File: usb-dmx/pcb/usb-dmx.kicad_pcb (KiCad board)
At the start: 2 copper layers, 25 x 35 mm, 22 parts, among them J1 USB_C_Receptacle_USB2.0_16P, J2 USB_A, SW1 PTS526_SM15_SMTR2_LFS, U1 IP4234CZ6, U2 ADP2108AUJ-3.3, U3 ESP32-S3-MINI-1U, U4 ST485E

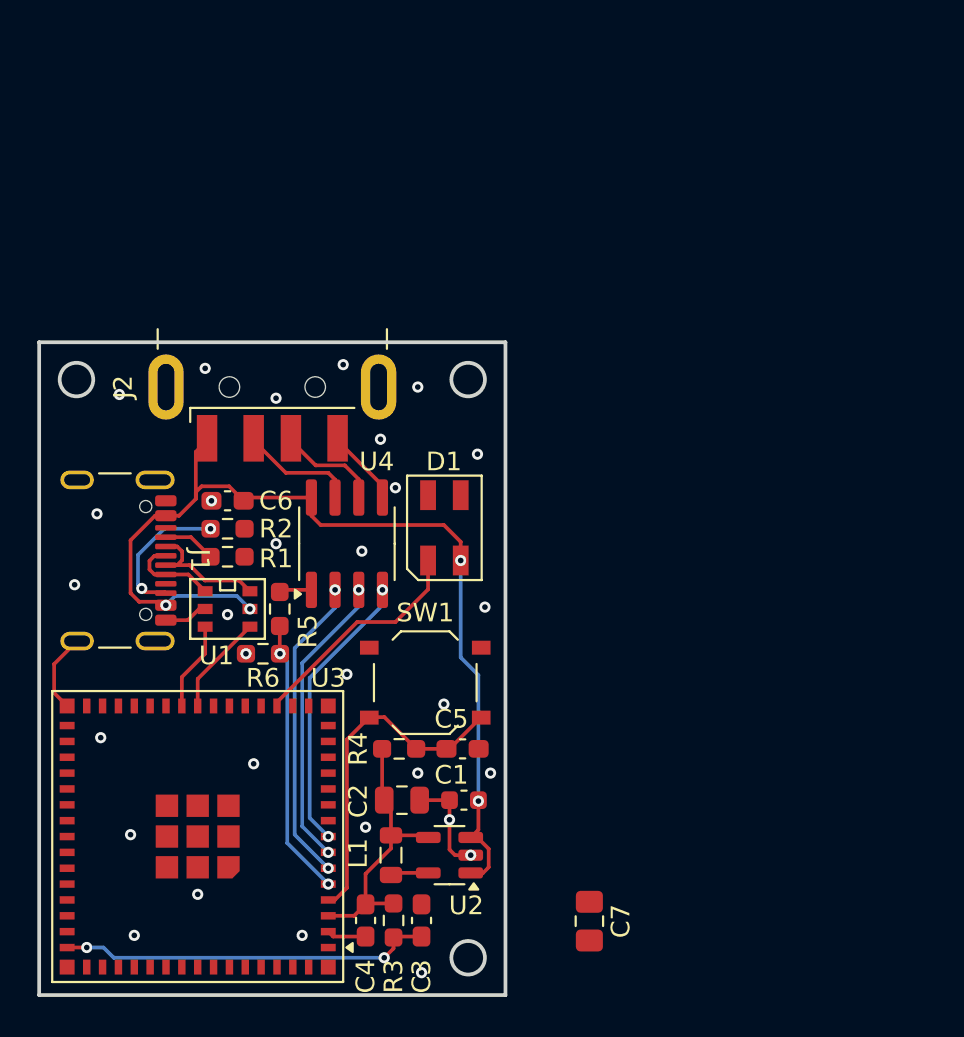
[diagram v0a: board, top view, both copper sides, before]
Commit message: creating pcb layout
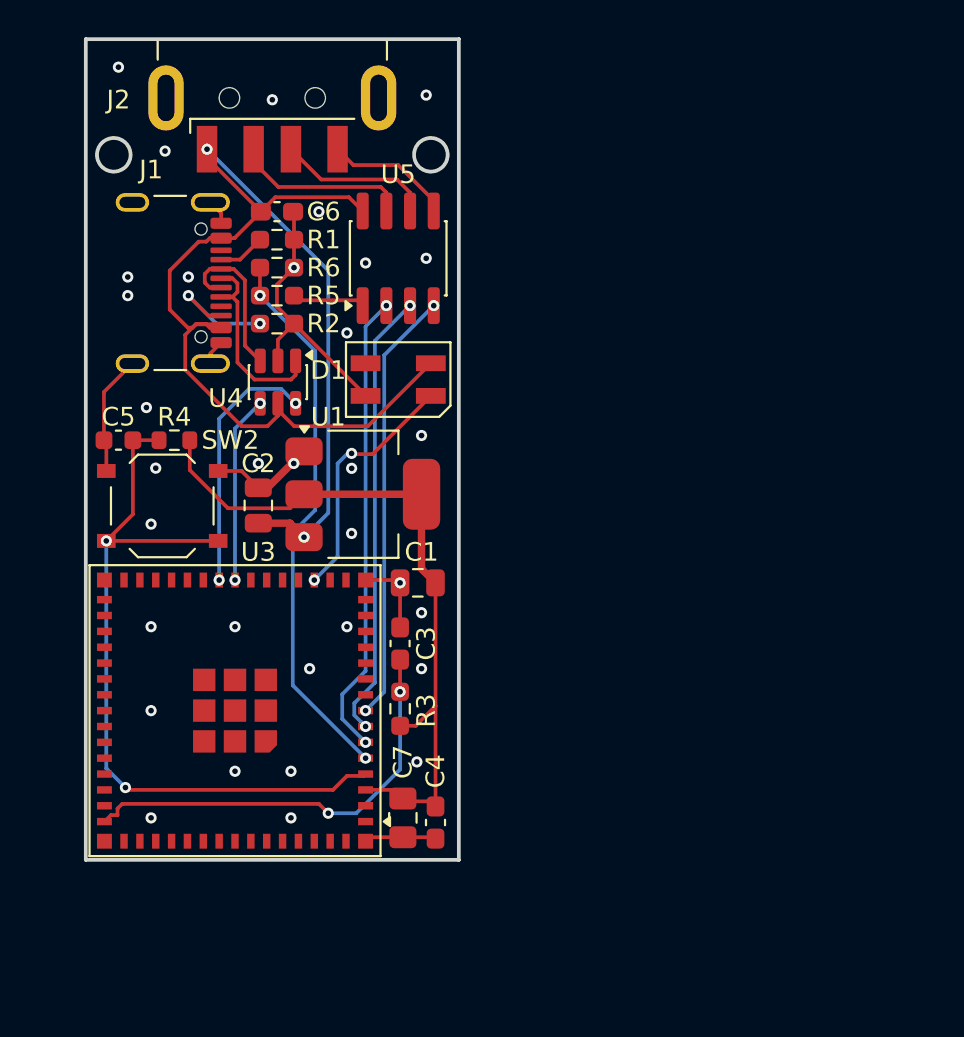
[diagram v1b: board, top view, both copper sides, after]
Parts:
- removed L1: 1uH, Inductor_SMD:L_0805_2012Metric
- removed SW1: PTS526_SM15_SMTR2_LFS, Button_Switch_SMD:SW_Push_1P1T_XKB_TS-1187A
- removed U2: ADP2108AUJ-3.3, Package_TO_SOT_SMD:TSOT-23-5
- added SW2: SW_Push, Button_Switch_SMD:SW_Push_1P1T_XKB_TS-1187A, F.Cu at (94.1, 68.8)
- added U5: MAX485E, Package_SO:SOP-8_3.76x4.96mm_P1.27mm, F.Cu at (106.8, 55.5)
- C1: value 4.7uF -> 22uF; footprint Capacitor_SMD:C_0603_1608Metric -> Capacitor_SMD:C_0805_2012Metric
- C2: value 10uF -> 22uF
- C5: footprint Capacitor_SMD:C_0603_1608Metric_Pad1.08x0.95mm_HandSolder -> Capacitor_SMD:C_0603_1608Metric
- R4: footprint Resistor_SMD:R_0603_1608Metric_Pad0.98x0.95mm_HandSolder -> Resistor_SMD:R_0603_1608Metric
- U1: value IP4234CZ6 -> AMS1117-3.3; footprint footprints:IP4234CZ6_SOT-457-6 -> Package_TO_SOT_SMD:SOT-223-3_TabPin2
- U4: value ST485E -> USBLC6-2SC6; footprint Package_SO:SOIC-8_3.9x4.9mm_P1.27mm -> Package_TO_SOT_SMD:SOT-23-6
- moved C5 24.8 mm to (91.8, 65.2), turned to 180 degrees
- moved R6 20.7 mm to (100.2, 56.0), turned to 0 degrees
- moved R4 20.5 mm to (94.8, 65.2), turned to 180 degrees
- moved C2 17.6 mm to (99.2, 68.8), turned to 90 degrees
- moved R1 17.2 mm to (100.2, 54.5)
- moved R5 16.8 mm to (100.2, 57.5), turned to 0 degrees
- moved C6 15.7 mm to (100.2, 53.0), turned to 0 degrees
- moved J2 15.5 mm to (100.0, 40.0)
- moved J1 15.2 mm to (93.6, 56.8)
- moved C3 14.9 mm to (106.8, 76.2)
- moved C1 11.9 mm to (107.8, 72.9)
- moved C7 11.4 mm to (107.0, 85.5)
- moved R3 11.4 mm to (106.8, 79.7), turned to 90 degrees
- moved R2 11.3 mm to (100.2, 59.0)
- moved U1 9.51 mm to (104.8, 68.2)
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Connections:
- C1 pad 1: VCC_5V -> VCC_3.3V
- C2 pad 1: VCC_3.3V -> VCC_5V
- R5 pad 2: Net-(U4-RO) -> Net-(U5-RO)
- U1 pad 1: Net-(J1-D+-PadA6) -> GND
- U1 pad 2: GND -> VCC_3.3V
- U1 pad 3: D+ -> VCC_5V
- U4 pad 1: Net-(U4-RO) -> Net-(J1-D+-PadA6)
- U4 pad 2: 2 -> GND
- U4 pad 3: 3 -> Net-(J1-D--PadA7)
- U4 pad 4: 4 -> D-
- U4 pad 5: GND -> VCC_5V
- U4 pad 6: DMX+ -> D+
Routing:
- net GND: track 18.3 -> 45.0 mm, vias 30 -> 33
- net VCC_3.3V: track 14.9 -> 38.7 mm
- net 0: track 18.3 -> 40.3 mm, vias 0 -> 2
- net VCC_5V: track 54.2 -> 70.6 mm, vias 4 -> 2
- net 1: track 14.9 -> 29.6 mm
- net D+: track 4.77 -> 13.7 mm, vias 0 -> 2
- net 2: track 16.6 -> 24.9 mm
- net 3: track 15.9 -> 24.0 mm
- net 4: track 15.3 -> 23.2 mm
- net Net-(J1-D+-PadA6): track 4.92 -> 10.4 mm
- net D-: track 5.41 -> 10.0 mm, vias 0 -> 2
- net Net-(U5-RO): track 0.00 -> 3.80 mm
- net Net-(U3-EN): track 20.0 -> 23.5 mm
- net DMX-: track 6.19 -> 9.48 mm
- net DMX+: track 5.47 -> 8.34 mm
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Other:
- board size 25 x 35 mm -> 20 x 44 mm
- board text added: "${REFERENCE}"
- board text added: "TRANCE USB-DMX Rev: 1.2"
- board text removed: "TRANCE USB-DMX Rev: 1.1"

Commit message: updating documentation
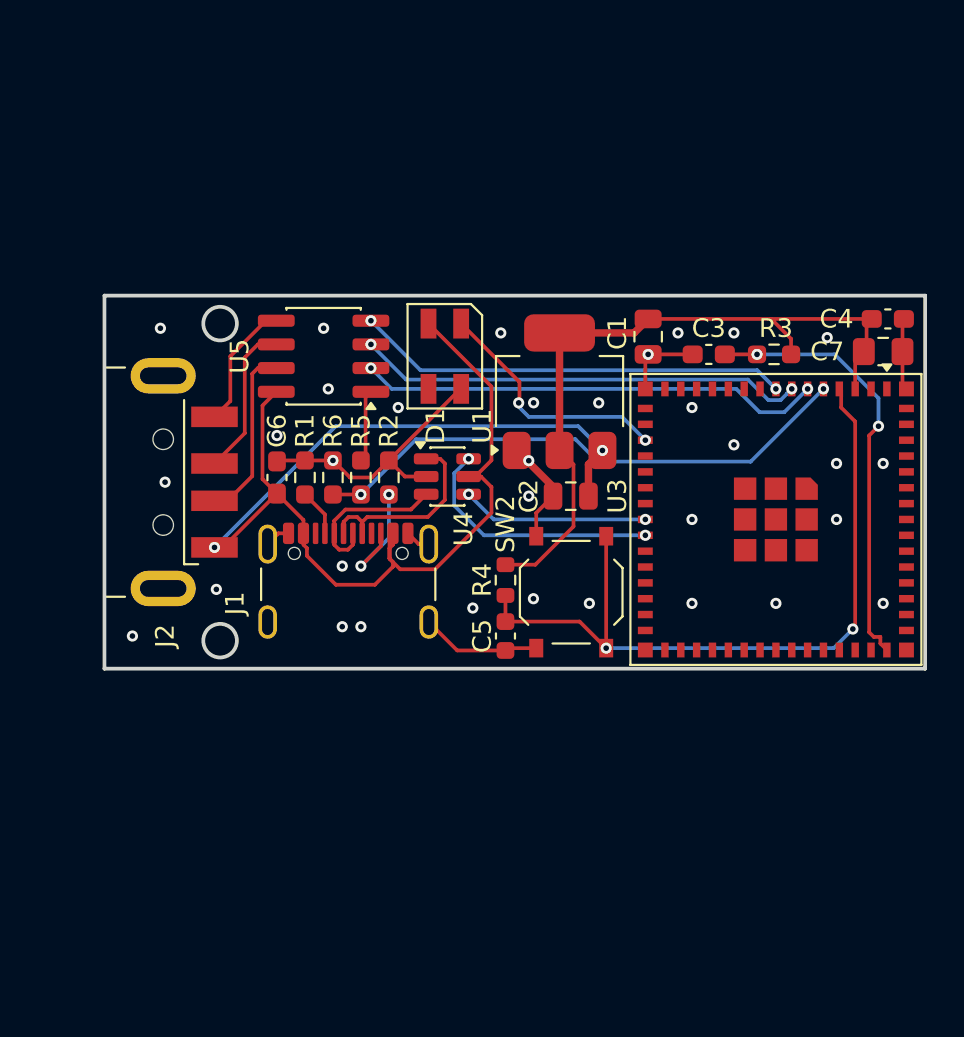
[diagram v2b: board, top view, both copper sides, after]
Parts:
- moved C4 36.3 mm to (133.0, 58.8), turned to 0 degrees
- moved C7 35.9 mm to (132.8, 60.5), turned to 0 degrees
- moved U3 30.8 mm to (127.0, 69.5), turned to -90 degrees
- moved J2 30.3 mm to (87.2, 67.5), turned to 180 degrees
- moved R3 27.6 mm to (126.9, 60.6), turned to 180 degrees
- moved C5 23.3 mm to (112.5, 75.8), turned to -90 degrees
- moved C3 22.7 mm to (123.4, 60.6), turned to 180 degrees
- moved SW2 22.4 mm to (116.0, 73.4), turned to 90 degrees
- moved J1 20.1 mm to (104.1, 73.9), turned to 0 degrees
- moved R4 19.3 mm to (112.5, 72.8), turned to -90 degrees
- moved C1 18.1 mm to (120.2, 59.7), turned to -90 degrees
- moved C2 16.8 mm to (116.0, 68.2), turned to 180 degrees
- moved C6 14.2 mm to (100.2, 67.2), turned to 90 degrees
- moved R1 12.8 mm to (101.8, 67.2), turned to 90 degrees
- moved U1 11.9 mm to (115.4, 62.6), turned to 90 degrees
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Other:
- board size 20 x 44 mm -> 44 x 20 mm
